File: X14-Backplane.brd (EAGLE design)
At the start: 88.9 x 140.2 mm, 28 parts, among them J2 PXC-PTSM-04-RA-1778641, J3 PXC-8-RA-1778683, J8 PXC-8-RA-1778683

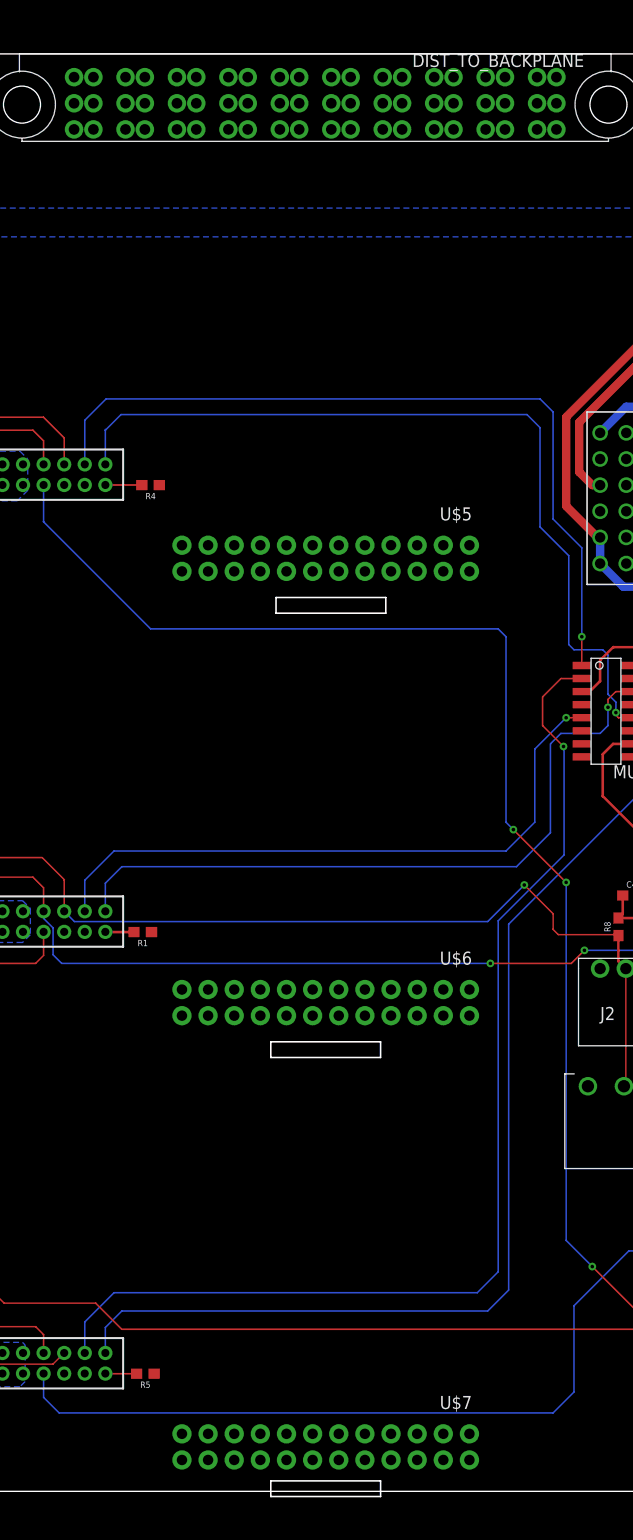
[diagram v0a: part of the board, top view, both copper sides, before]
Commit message: X14-Backplane 12/4
This is the most up to date version as of 12/4/2021
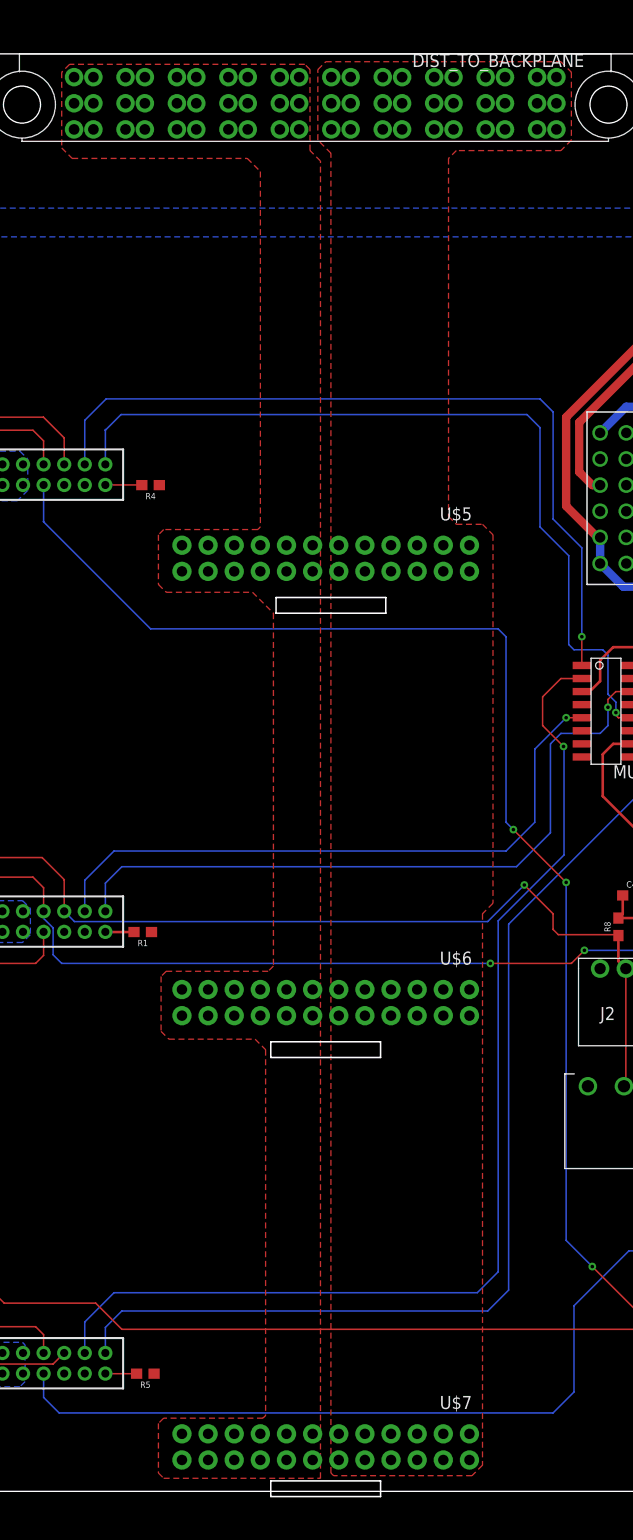
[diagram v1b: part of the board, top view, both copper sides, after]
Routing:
- added copper zone on layer 1, net 12V
- added copper zone on layer 1, net 12VGND
